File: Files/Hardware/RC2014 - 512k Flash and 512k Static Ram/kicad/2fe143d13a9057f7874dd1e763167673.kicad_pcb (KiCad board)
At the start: 2 copper layers, 102.5 x 45.7 mm, 18 parts, among them CON1 RC2014, IC1 74HCT670N, IC2 74HCT670N, IC3 74HCT139N, IC4 74HCT138N, IC5 74HCT74N, IC6 39SF040, IC7 AS6C4008

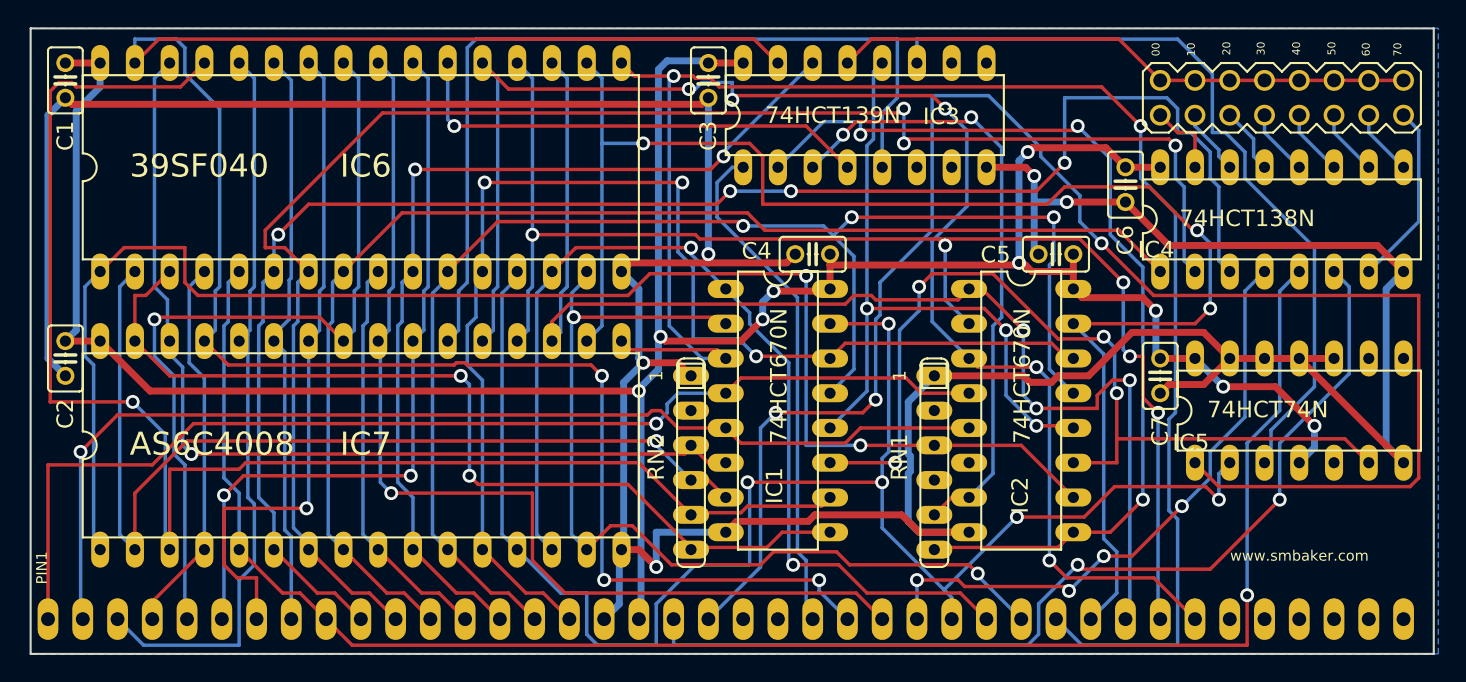
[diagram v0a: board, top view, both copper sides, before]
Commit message: Some changes
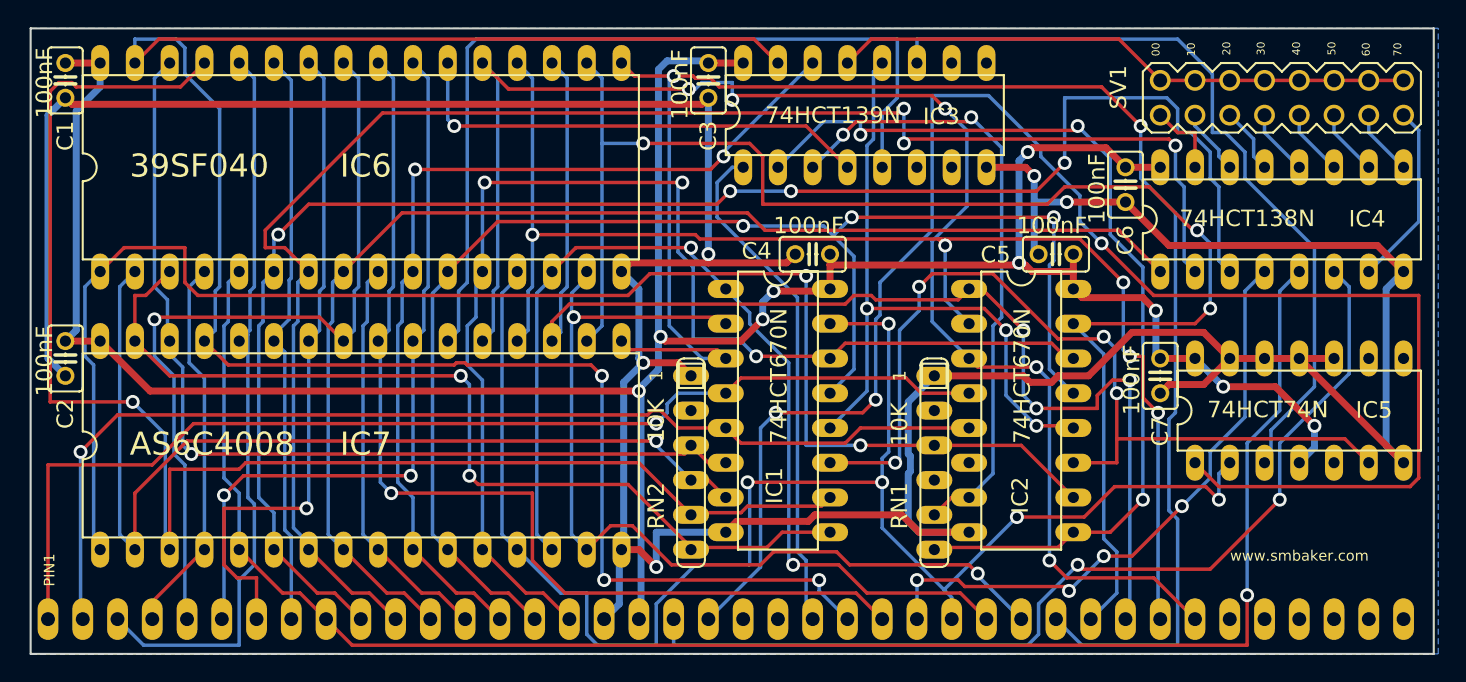
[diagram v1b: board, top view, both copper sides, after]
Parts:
- CON1: value RC2014 -> RC2014 Backplane
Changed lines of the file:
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@@
       (effects (font (size 1.27 1.27) (thickness 0.15)))
     )
-    (fp_text value RC2014 (at 0 0) (layer F.SilkS) hide
+    (fp_text value "RC2014 Backplane" (at 0 0) (layer F.SilkS) hide
       (effects (font (size 1.27 1.27) (thickness 0.15)))
     )
@@
       (effects (font (size 1.2065 1.2065) (thickness 0.127)) (justify right top))
     )
-    (fp_text value 100nF (at -2.286 2.794 90) (layer F.Fab) hide
+    (fp_text value 100nF (at -2.3826 2.2351 90) (layer F.SilkS)
       (effects (font (size 1.2065 1.2065) (thickness 0.12065)) (justify right top))
     )
@@
       (effects (font (size 1.2065 1.2065) (thickness 0.127)) (justify right top))
     )
-    (fp_text value 100nF (at -2.286 2.794 90) (layer F.Fab) hide
+    (fp_text value 100nF (at -2.3826 2.2351 90) (layer F.SilkS)
       (effects (font (size 1.2065 1.2065) (thickness 0.12065)) (justify right top))
     )
@@
       (effects (font (size 1.2065 1.2065) (thickness 0.127)) (justify right top))
     )
-    (fp_text value 100nF (at -2.286 2.794 90) (layer F.Fab) hide
+    (fp_text value 100nF (at -2.286 2.794 90) (layer F.SilkS)
       (effects (font (size 1.2065 1.2065) (thickness 0.12065)) (justify right top))
     )
@@
       (effects (font (size 1.2065 1.2065) (thickness 0.127)) (justify right top))
     )
-    (fp_text value 100nF (at -2.286 2.794) (layer F.Fab) hide
+    (fp_text value 100nF (at -2.286 2.794) (layer F.SilkS)
       (effects (font (size 1.2065 1.2065) (thickness 0.12065)) (justify right top))
     )
@@
       (effects (font (size 1.2065 1.2065) (thickness 0.127)) (justify right top))
     )
-    (fp_text value 100nF (at -2.286 2.794) (layer F.Fab) hide
+    (fp_text value 100nF (at -2.286 2.794) (layer F.SilkS)
       (effects (font (size 1.2065 1.2065) (thickness 0.12065)) (justify right top))
     )
@@
     (at 188.6711 96.1086)
     (descr "<b>Dual In Line Package</b>")
-    (fp_text reference IC4 (at -10.541 2.921) (layer F.SilkS)
+    (fp_text reference IC4 (at 4.8769 0.6654) (layer F.SilkS)
       (effects (font (size 1.2065 1.2065) (thickness 0.12065)) (justify left bottom))
     )
@@
     (at 189.9411 110.0786)
     (descr "<b>Dual In Line Package</b>")
-    (fp_text reference IC5 (at -9.271 3.048) (layer F.SilkS)
+    (fp_text reference IC5 (at 4.1149 0.6654) (layer F.SilkS)
       (effects (font (size 1.2065 1.2065) (thickness 0.12065)) (justify left bottom))
     )
@@
     (at 188.6711 87.2186 180)
     (descr "<b>PIN HEADER</b>")
-    (fp_text reference SV1 (at -10.16 -2.921 180) (layer F.SilkS) hide
+    (fp_text reference SV1 (at 12.6491 2.3826 90) (layer F.SilkS)
       (effects (font (size 1.2065 1.2065) (thickness 0.127)) (justify right top))
     )
@@
       (effects (font (size 1.2065 1.2065) (thickness 0.127)) (justify right top))
     )
-    (fp_text value 100nF (at -2.286 2.794 90) (layer F.Fab) hide
+    (fp_text value 100nF (at -2.286 2.794 90) (layer F.SilkS)
       (effects (font (size 1.2065 1.2065) (thickness 0.12065)) (justify right top))
     )
@@
     (at 163.2711 113.8886 270)
     (descr "<b>Single In Line</b>")
-    (fp_text reference RN1 (at -2.1286 3.2511 270) (layer F.SilkS)
+    (fp_text reference RN1 (at 1.4274 3.2511 270) (layer F.SilkS)
       (effects (font (size 1.2065 1.2065) (thickness 0.127)) (justify right top))
     )
-    (fp_text value 10K (at -0.635 -1.27 90) (layer F.Fab) hide
+    (fp_text value 10K (at -4.4146 3.2511 90) (layer F.SilkS)
       (effects (font (size 1.2065 1.2065) (thickness 0.12065)) (justify right top))
     )
@@
     (at 145.4911 113.8886 270)
     (descr "<b>Single In Line</b>")
-    (fp_text reference RN2 (at -2.1286 3.2511 270) (layer F.SilkS)
+    (fp_text reference RN2 (at 1.4274 3.2511 270) (layer F.SilkS)
       (effects (font (size 1.2065 1.2065) (thickness 0.127)) (justify right top))
     )
-    (fp_text value 10K (at -0.635 -1.27 90) (layer F.Fab) hide
+    (fp_text value 10K (at -4.6686 3.2511 90) (layer F.SilkS)
       (effects (font (size 1.2065 1.2065) (thickness 0.12065)) (justify right top))
     )
@@
       (effects (font (size 1.2065 1.2065) (thickness 0.127)) (justify right top))
     )
-    (fp_text value 100nF (at -2.286 2.794 90) (layer F.Fab) hide
+    (fp_text value 100nF (at -2.286 2.794 90) (layer F.SilkS)
       (effects (font (size 1.2065 1.2065) (thickness 0.12065)) (justify right top))
     )
@@
   (gr_line (start 199.7711 82.1486) (end 97.2311 82.1486) (layer Edge.Cuts) (width 0.15))
   (gr_line (start 97.2311 82.1486) (end 97.2311 127.8586) (layer Edge.Cuts) (width 0.15))
-  (gr_text PIN1 (at 98.5011 122.7786 90) (layer F.SilkS)
+  (gr_text PIN1 (at 99.06 122.936 90) (layer F.SilkS)
     (effects (font (size 0.77216 0.77216) (thickness 0.065024)) (justify left bottom))
   )
